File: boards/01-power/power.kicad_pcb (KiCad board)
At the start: 8 copper layers, 50 x 50 mm, 46 parts, among them J1 CONN_DF40_100P_F, J2 USB_C_Receptacle_USB2.0_16P, J3 TC2030, J4 TC2030, P1 MAG_RB1_125BAG1A, SW1 SW_BOOT, SW2 SW_BOOT, U1 USBLC6-2P6, U2 AP63203WU, U3 STM32F405RGTx, U4 PMIC_TPS2372_4RGWR, Y1 16Mhz

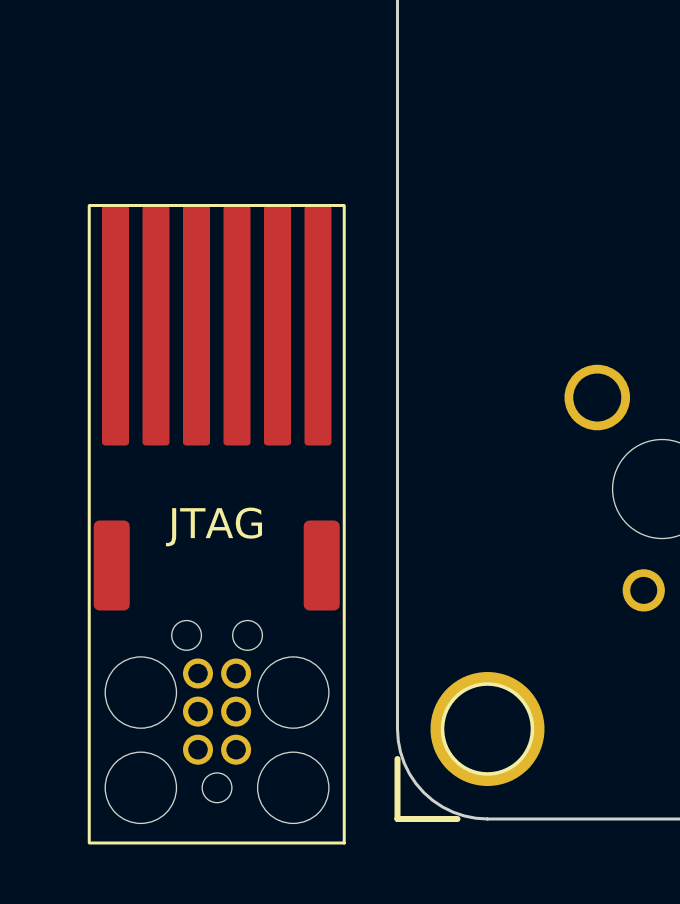
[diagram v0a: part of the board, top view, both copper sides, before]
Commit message: feat: outline
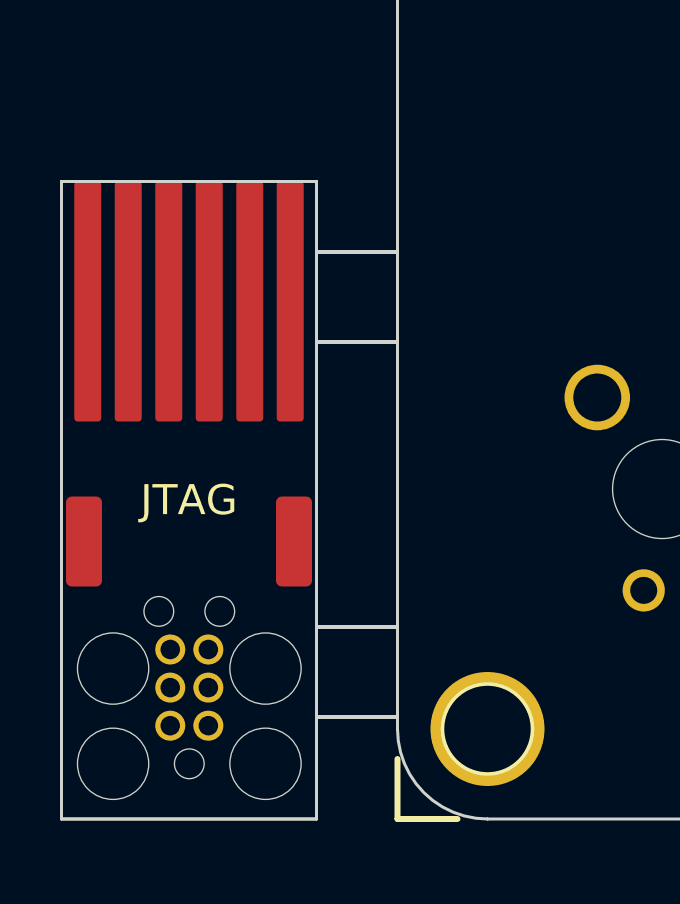
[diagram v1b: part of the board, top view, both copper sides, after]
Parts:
- moved JTAG 1.22 mm to (43.0, 96.2)
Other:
- board size 50 x 50 mm -> 61.2 x 50 mm
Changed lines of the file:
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@@
 	)
 	(footprint "Woki:CONN_TC2030_JTAG_PROBE"
+		(locked yes)
 		(layer "F.Cu")
-		(at 43.975 97.05 180)
+		(at 43.05 96.25 180)
 		(descr "Generated from CONN_TC2030_JTAG.kicad_mod; TC2030 pitch 1.27 mm, C5157236 tip 0.80 mm leaves 0.47 mm between tips, barrel 1.20 mm leaves 0.07 mm between barrels")
 		(tags "tc2030 jtag swd pogo probe card-edge")
@@
 		(layer "F.SilkS")
 	)
+	(gr_rect
+		(start 38.8 78.75)
+		(end 47.3 100)
+		(radius 1)
+		(stroke
+			(width 0.1)
+			(type default)
+		)
+		(fill no)
+		(layer "Edge.Cuts")
+	)
+	(gr_line
+		(start 47.3 81.1)
+		(end 50 81.1)
+		(stroke
+			(width 0.1)
+			(type default)
+		)
+		(layer "Edge.Cuts")
+	)
+	(gr_rect
+		(start 47.3 81.1)
+		(end 50 84.1)
+		(stroke
+			(width 0.1)
+			(type default)
+		)
+		(fill no)
+		(layer "Edge.Cuts")
+	)
+	(gr_line
+		(start 47.3 84.1)
+		(end 50 84.1)
+		(stroke
+			(width 0.1)
+			(type default)
+		)
+		(layer "Edge.Cuts")
+	)
+	(gr_line
+		(start 47.3 93.6)
+		(end 50 93.6)
+		(stroke
+			(width 0.1)
+			(type default)
+		)
+		(layer "Edge.Cuts")
+	)
+	(gr_rect
+		(start 47.3 93.6)
+		(end 50 96.6)
+		(stroke
+			(width 0.1)
+			(type default)
+		)
+		(fill no)
+		(layer "Edge.Cuts")
+	)
+	(gr_line
+		(start 47.3 96.6)
+		(end 50 96.6)
+		(stroke
+			(width 0.1)
+			(type default)
+		)
+		(layer "Edge.Cuts")
+	)
 	(gr_line
